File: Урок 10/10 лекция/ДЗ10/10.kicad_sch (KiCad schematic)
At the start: 22 parts

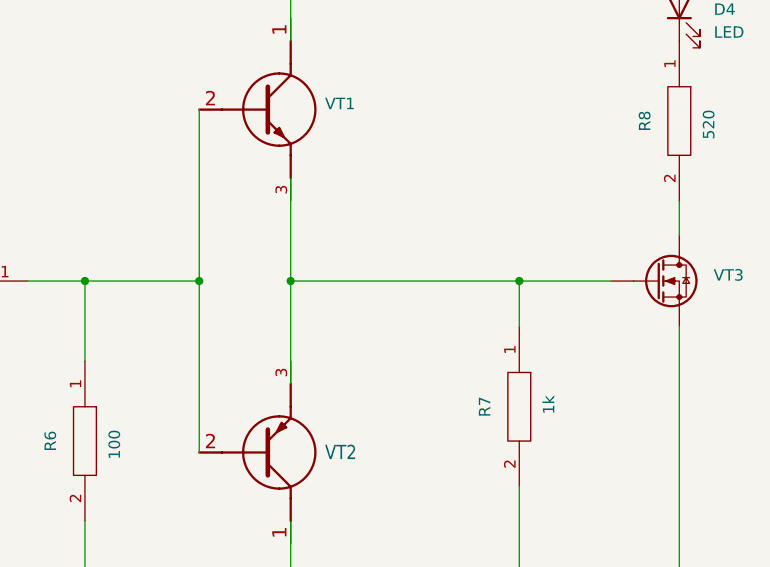
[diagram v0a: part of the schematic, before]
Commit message: 13
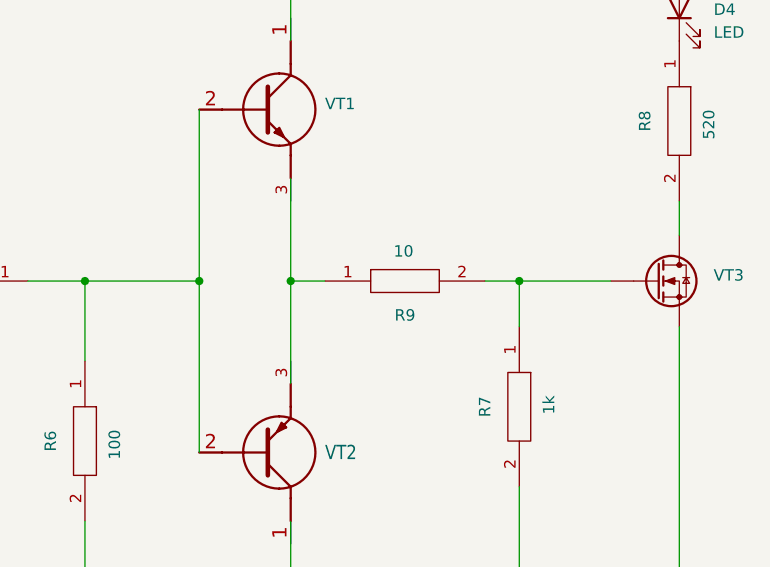
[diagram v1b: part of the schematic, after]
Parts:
- added R9: 10, RESAD2700W60L1100D400, symbol My_Lib:R - CF100-3K3-J-TB-070-62
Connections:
- net at VT1.3 (A), VT2.3 (A): now also R9.1; no longer R7.1, VT3.G
- new net: R7.1, R9.2, VT3.G
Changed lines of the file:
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@@
 	(wire
 		(pts
-			(xy 208.28 95.25) (xy 233.68 95.25)
+			(xy 208.28 95.25) (xy 212.09 95.25)
 		)
 		(stroke
@@
 	(wire
 		(pts
+			(xy 229.87 95.25) (xy 233.68 95.25)
+		)
+		(stroke
+			(width 0)
+			(type default)
+		)
+	)
+	(wire
+		(pts
 			(xy 52.07 38.1) (xy 52.07 35.56)
 		)
@@
 					(unit 1)
 				)
+			)
+		)
+	)
+	(symbol
+		(lib_id "My_Lib:R - CF100-3K3-J-TB-070-62")
+		(at 212.09 95.25 0)
+		(unit 1)
+		(exclude_from_sim no)
+		(in_bom yes)
+		(on_board yes)
+		(dnp no)
+		(property "Reference" "R9"
+			(at 220.98 99.06 0)
+			(effects
+				(font
+					(size 1.27 1.27)
+				)
+			)
+		)
+		(property "Value" "10"
+			(at 219.71 91.948 0)
+			(effects
+				(font
+					(size 1.27 1.27)
+				)
+				(justify left)
+			)
+		)
+		(property "Footprint" "RESAD2700W60L1100D400"
+			(at 226.06 93.98 0)
+			(effects
+				(font
+					(size 1.27 1.27)
+				)
+				(justify left)
+				(hide yes)
+			)
+		)
+		(property "Datasheet" ""
+			(at 226.06 96.52 0)
+			(effects
+				(font
+					(size 1.27 1.27)
+				)
+				(justify left)
+				(hide yes)
+			)
+		)
+		(property "Description" "CF100-3K3-J-TB-070-62 CARBON FILM FIXED RESISTOR, 1.0(1W)"
+			(at 212.09 95.25 0)
+			(effects
+				(font
+					(size 1.27 1.27)
+				)
+				(hide yes)
+			)
+		)
+		(property "Description_1" "CARBON FILM FIXED RESISTOR, 1.0(1W)"
+			(at 226.06 99.06 0)
+			(effects
+				(font
+					(size 1.27 1.27)
+				)
+				(justify left)
+				(hide yes)
+			)
+		)
+		(property "Height" ""
+			(at 226.06 101.6 0)
+			(effects
+				(font
+					(size 1.27 1.27)
+				)
+				(justify left)
+				(hide yes)
+			)
+		)
+		(property "Manufacturer_Name" "HKR"
+			(at 226.06 104.14 0)
+			(effects
+				(font
+					(size 1.27 1.27)
+				)
+				(justify left)
+				(hide yes)
+			)
+		)
+		(property "Manufacturer_Part_Number" "CF100-3K3-J-TB-070-62"
+			(at 226.06 106.68 0)
+			(effects
+				(font
+					(size 1.27 1.27)
+				)
+				(justify left)
+				(hide yes)
+			)
+		)
+		(property "Mouser Part Number" ""
+			(at 226.06 109.22 0)
+			(effects
+				(font
+					(size 1.27 1.27)
+				)
+				(justify left)
+				(hide yes)
+			)
+		)
+		(property "Mouser Price/Stock" ""
+			(at 226.06 111.76 0)
+			(effects
+				(font
+					(size 1.27 1.27)
+				)
+				(justify left)
+				(hide yes)
+			)
+		)
+		(property "Arrow Part Number" ""
+			(at 226.06 114.3 0)
+			(effects
+				(font
+					(size 1.27 1.27)
+				)
+				(justify left)
+				(hide yes)
+			)
+		)
+		(property "Arrow Price/Stock" ""
+			(at 226.06 116.84 0)
+			(effects
+				(font
+					(size 1.27 1.27)
+				)
+				(justify left)
+				(hide yes)
+			)
+		)
+		(pin "1"
+		)
+		(pin "2"
+		)
+		(instances
+			(project "10"
+				(path "/a16ced28-de46-4a09-9281-b6aa8ba3a935"
+					(reference "R9")
+					(unit 1)
+				)
